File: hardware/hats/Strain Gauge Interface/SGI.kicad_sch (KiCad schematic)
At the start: 95 parts, among them IC1 ADC124S051CIMM_NOPB, J1 JST-XA, J10 JST-XA, J11 JST-XA, J12 JST-XA, J13 JST-XA, J14 JST-XA, J15 JST-XA, J16 JST-XA, J17 JST-XA, J2 S03B-XASK-1, J3 S03B-XASK-1, J4 S03B-XASK-1, J5 S03B-XASK-1, J6 S03B-XASK-1, J7 S03B-XASK-1, J8 S03B-XASK-1, J9 S03B-XASK-1, U1 REF5025IDGKR, U10 INA333xxDGK, U11 INA333xxDGK, U12 INA333xxDGK, U13 TME-1205S, U14 ISO1042BQDWVRQ1, U15 ESP32-S2-DEVKITC-1, U2 POPA994QDBVRQ1, U3 LMR50410Y5FQDBVRQ1, U4 POPA994QDBVRQ1, U5 INA333xxDGK, U6 INA333xxDGK, U7 INA333xxDGK, U8 INA333xxDGK, U9 INA333xxDGK

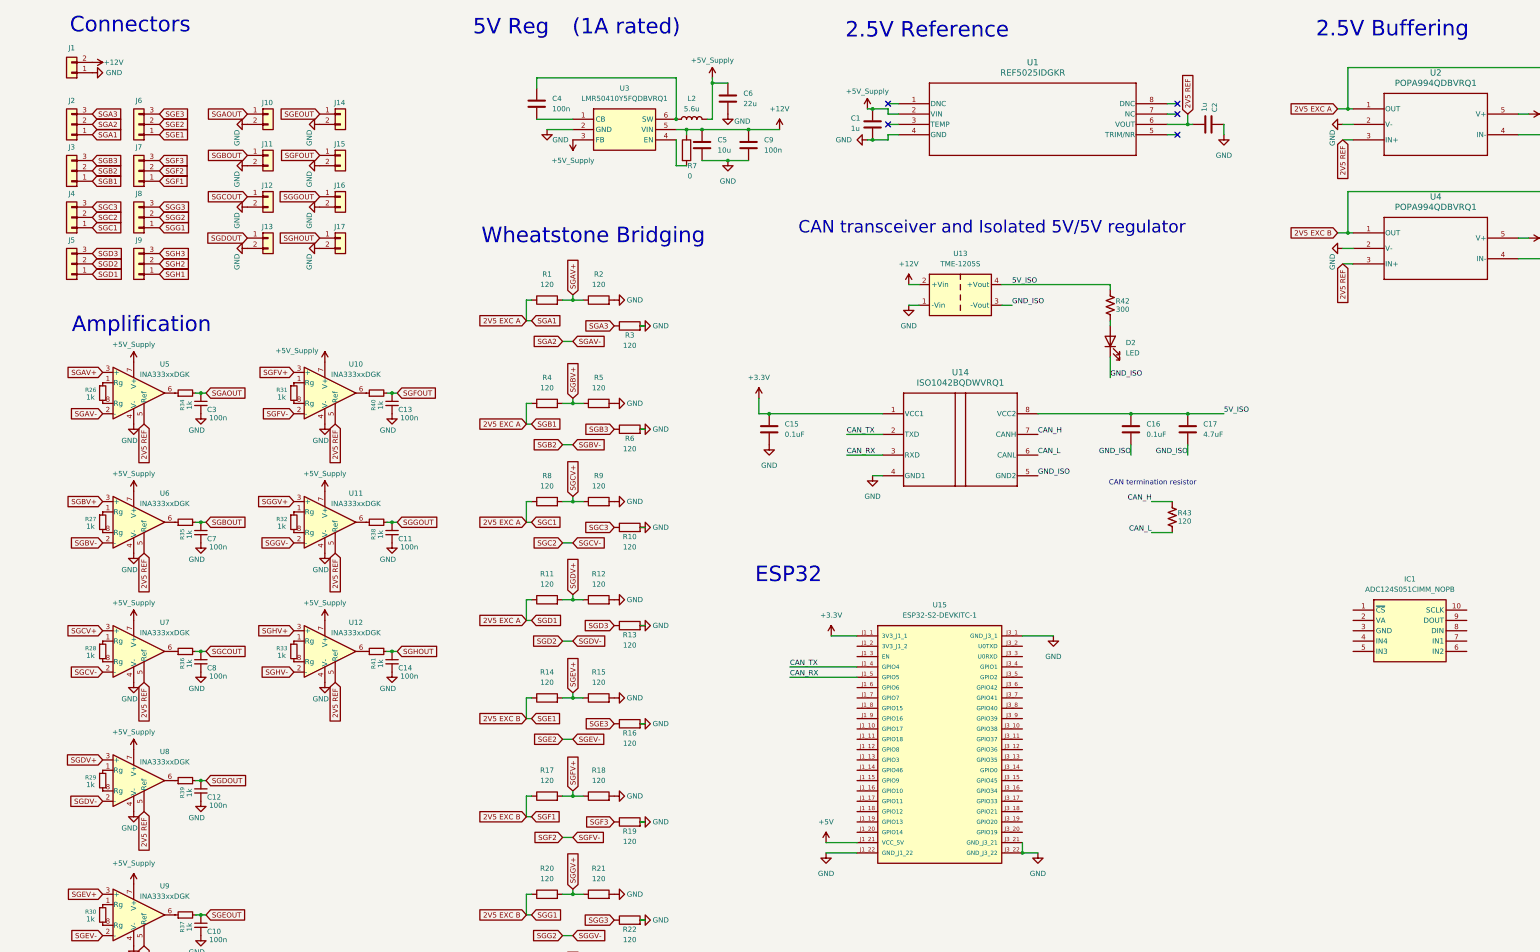
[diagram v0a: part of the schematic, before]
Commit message: hats
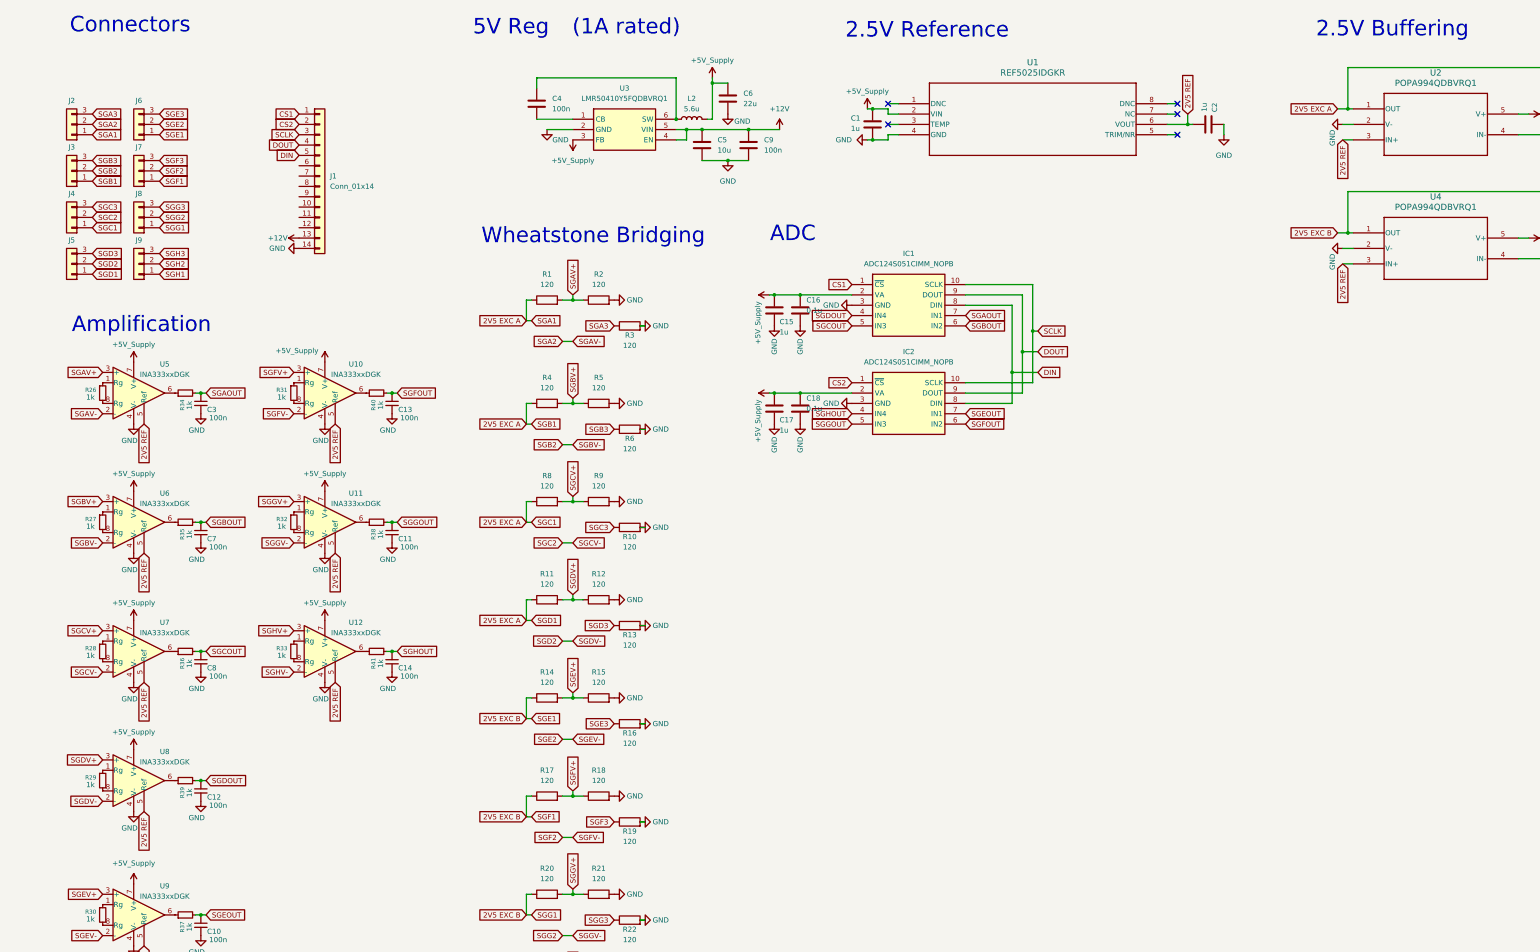
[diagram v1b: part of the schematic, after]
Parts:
- removed D2: LED, LED_SMD:LED_0603_1608Metric_Pad1.05x0.95mm_HandSolder, symbol Device:LED
- removed J1, J10, J11, J12, J13, J14, J15, J16, J17: JST-XA, Custom_MSM:Connector_JST-XA_2POS, symbol Custom_MSM:Connector_JST-XA_2POS
- removed R42: 300, Resistor_SMD:R_0603_1608Metric_Pad0.98x0.95mm_HandSolder, symbol Device:R_US
- removed R43: 120, Resistor_SMD:R_0603_1608Metric_Pad0.98x0.95mm_HandSolder, symbol Device:R_US
- removed R7: 0, Resistor_SMD:R_0603_1608Metric, symbol Device:R
- removed U13: TME-1205S, Converter_DCDC:Converter_DCDC_TRACO_TME_03xxS_05xxS_12xxS_Single_THT, symbol Converter_DCDC:TME-1205S
- removed U14: ISO1042BQDWVRQ1, Personal:DWV0008A-IPC_A, symbol ISO1042B:ISO1042BQDWVRQ1
- removed U15: ESP32-S2-DEVKITC-1, Personal:MODULE_ESP32-S2-DEVKITC-1, symbol ESP32-S2-DEVKITC-1:ESP32-S2-DEVKITC-1
- added C18: 0.1u, Capacitor_SMD:C_0603_1608Metric, symbol Device:C
- added IC2: ADC124S051CIMM_NOPB, customFootprints:SOP50P490X110-10N, symbol ADC124S051CIMM_NOPB:ADC124S051CIMM_NOPB
- added J1: Conn_01x14, Connector_JST:JST_XA_S14B-XASK-1_1x14_P2.50mm_Horizontal, symbol Connector_Generic:Conn_01x14
- C1, C10, C11, C12, C13, C14, C2, C3, C7, C8: footprint (none) -> Capacitor_SMD:C_0603_1608Metric
- C15: value 0.1uF -> 1u; footprint Capacitor_SMD:C_0603_1608Metric_Pad1.08x0.95mm_HandSolder -> Capacitor_SMD:C_0603_1608Metric
- C16: value 0.1uF -> 0.1u; footprint Capacitor_SMD:C_0603_1608Metric_Pad1.08x0.95mm_HandSolder -> Capacitor_SMD:C_0603_1608Metric
- C17: value 4.7uF -> 1u; footprint Capacitor_SMD:C_0603_1608Metric_Pad1.08x0.95mm_HandSolder -> Capacitor_SMD:C_0603_1608Metric
- IC1: footprint SOP50P490X110-10N -> customFootprints:SOP50P490X110-10N
- L2: footprint Inductor_SMD:L_0603_1608Metric -> customFootprints:Shielded_Inductor_SMD_7265
- R1, R10, R11, R12, R13, R14, R15, R16, R17, R18, R19, R2, R20, R21, R22, R23, R24, R25, R26, R27, R28, R29, R3, R30, R31, R32, R33, R34, R35, R36, R37, R38, R39, R4, R40, R41, R5, R6, R8, R9: footprint (none) -> Resistor_SMD:R_0603_1608Metric
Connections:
- net +3.3V is gone; now on net +5V_Supply: C15.1
- net 5V_ISO is gone; now on net +5V_Supply: C16.1, C17.1
- net GND_ISO is gone; now on net GND: C16.2, C17.2
- net +12V: now also U3.4 (EN), J1.13 (Pin_13)
- net +5V_Supply: now also IC1.2 (VA), C18.1, IC2.2 (VA)
- net GND: now also IC1.3 (GND), C18.2, IC2.3 (GND), J1.14 (Pin_14)
- net SGAOUT: now also IC1.7 (IN1)
- net SGBOUT: now also IC1.6 (IN2)
- net SGCOUT: now also IC1.5 (IN3)
- net SGDOUT: now also IC1.4 (IN4)
- net SGEOUT: now also IC2.7 (IN1)
- net SGFOUT: now also IC2.6 (IN2)
- net SGGOUT: now also IC2.5 (IN3)
- net SGHOUT: now also IC2.4 (IN4)
- net CS1: now reaches IC1.1 (~{CS})
- net CS1: now also J1.1 (Pin_1)
- net SCLK: now reaches IC1.10 (SCLK)
- net SCLK: now also IC2.10 (SCLK), J1.3 (Pin_3)
- net DIN: now reaches IC1.8 (DIN)
- net DIN: now also IC2.8 (DIN), J1.5 (Pin_5)
- net DOUT: now reaches IC1.9 (DOUT)
- net DOUT: now also IC2.9 (DOUT), J1.4 (Pin_4)
- new net CS2: IC2.1 (~{CS}), J1.2 (Pin_2)
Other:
- note added: "ADC"
- note removed: "CAN termination resistor"
- note removed: "CAN transceiver and Isolated 5V/5V regulator"
- note removed: "ESP32"

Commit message: final ordered version
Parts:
- L2: footprint customFootprints:Shielded_Inductor_SMD_7265 -> Inductor_SMD:L_Wuerth_WE-TPC-3816
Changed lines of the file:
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@@
 			)
 		)
-		(property "Footprint" "customFootprints:Shielded_Inductor_SMD_7265"
+		(property "Footprint" "Inductor_SMD:L_Wuerth_WE-TPC-3816"
 			(at 172.72 48.26 0)
 			(hide yes)

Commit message: strain gauge hell
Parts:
- L2: footprint Inductor_SMD:L_Wuerth_WE-TPC-3816 -> CustomFootprints:WE-TPC_4828
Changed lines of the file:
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@@
 			)
 		)
-		(property "Footprint" "Inductor_SMD:L_Wuerth_WE-TPC-3816"
+		(property "Footprint" "CustomFootprints:WE-TPC_4828"
 			(at 172.72 48.26 0)
 			(hide yes)
